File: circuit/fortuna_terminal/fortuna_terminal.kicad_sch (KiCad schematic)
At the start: 10 parts

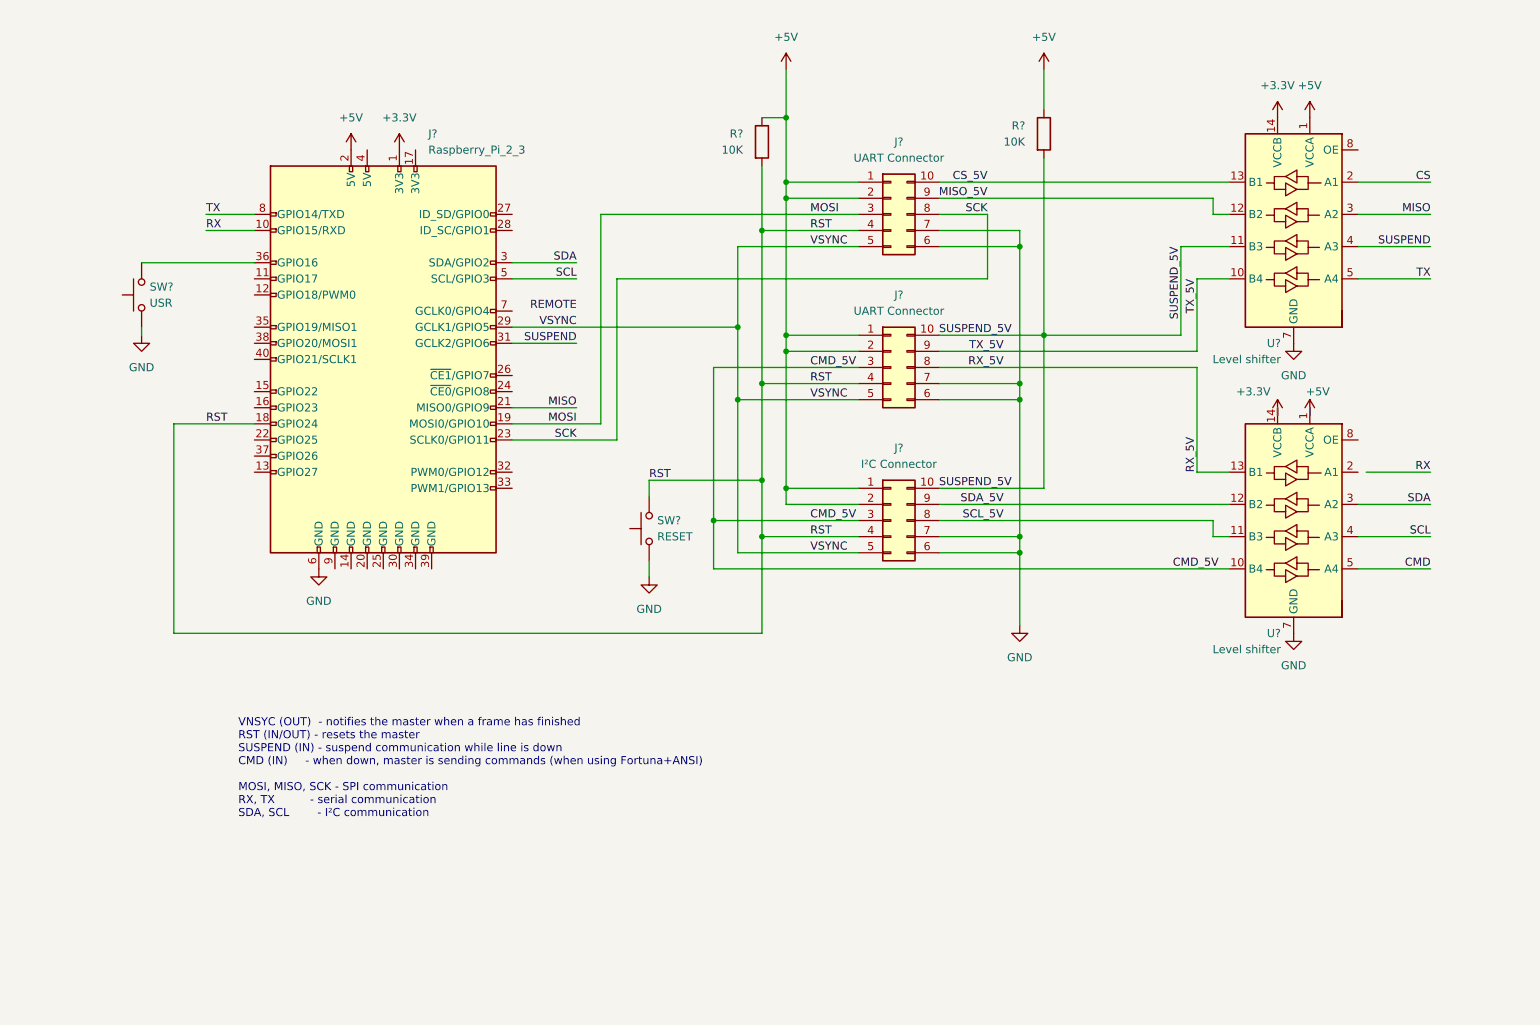
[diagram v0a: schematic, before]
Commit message: WIP
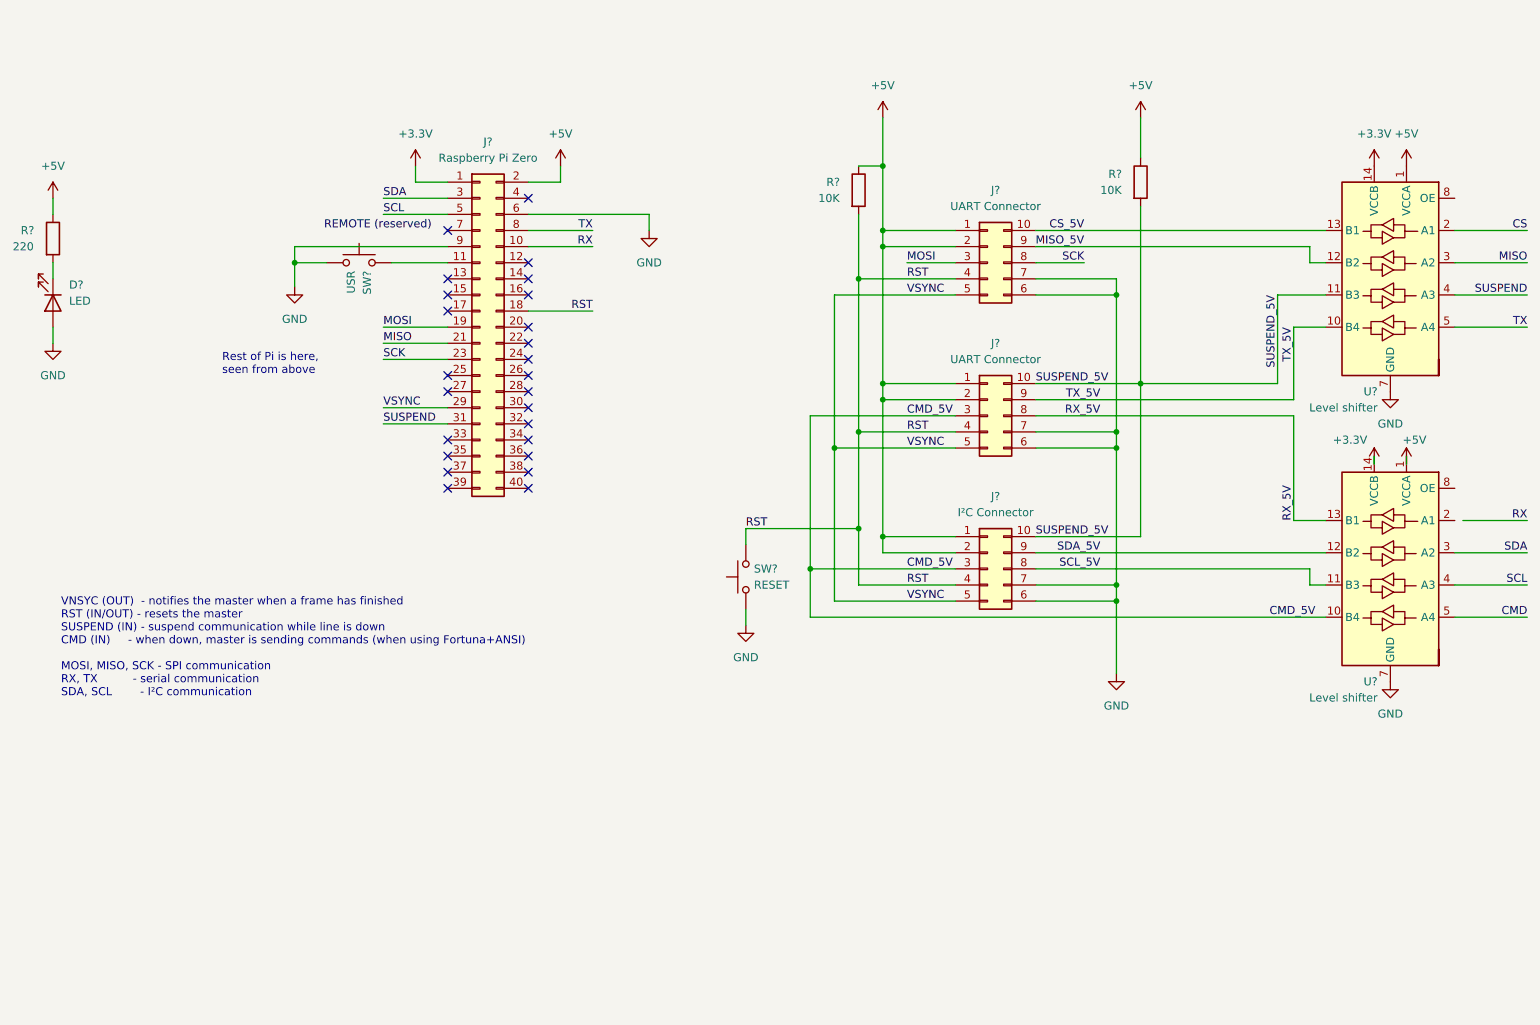
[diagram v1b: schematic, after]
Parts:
- removed J?: Raspberry_Pi_2_3, symbol Connector:Raspberry_Pi_2_3
- removed SW?: USR, symbol Switch:SW_Push
- added D?: LED, symbol Device:LED
- added J?: Raspberry Pi Zero, symbol Connector_Generic:Conn_02x20_Odd_Even
- added R?: 220, symbol Device:R
- added SW?: USR, symbol Switch:SW_Push
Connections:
- net +3.3V: now also J?.1 (Pin_1)
- net +5V: now also J?.2 (Pin_2), R?.1
- net GND: now also D?.2 (A), J?.6 (Pin_6), J?.9 (Pin_9), SW?.1
- net MISO: now also J?.21 (Pin_21)
- net MOSI: now also J?.19 (Pin_19)
- net RST: now also J?.18 (Pin_18)
- net RX: now also J?.10 (Pin_10)
- net SCK: now also J?.23 (Pin_23)
- net SCL: now also J?.5 (Pin_5)
- net SDA: now also J?.3 (Pin_3)
- net SUSPEND: now also J?.31 (Pin_31)
- net TX: now also J?.8 (Pin_8)
- net VSYNC: now also J?.29 (Pin_29)
- new net: J?.11 (Pin_11), SW?.2
- new net: D?.1 (K), R?.2
- no-connect marks 0 -> 25
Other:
- note added: "Rest of Pi is here, seen from above"
- moved on the sheet: J?, R?, SW?, U?

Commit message: WIP
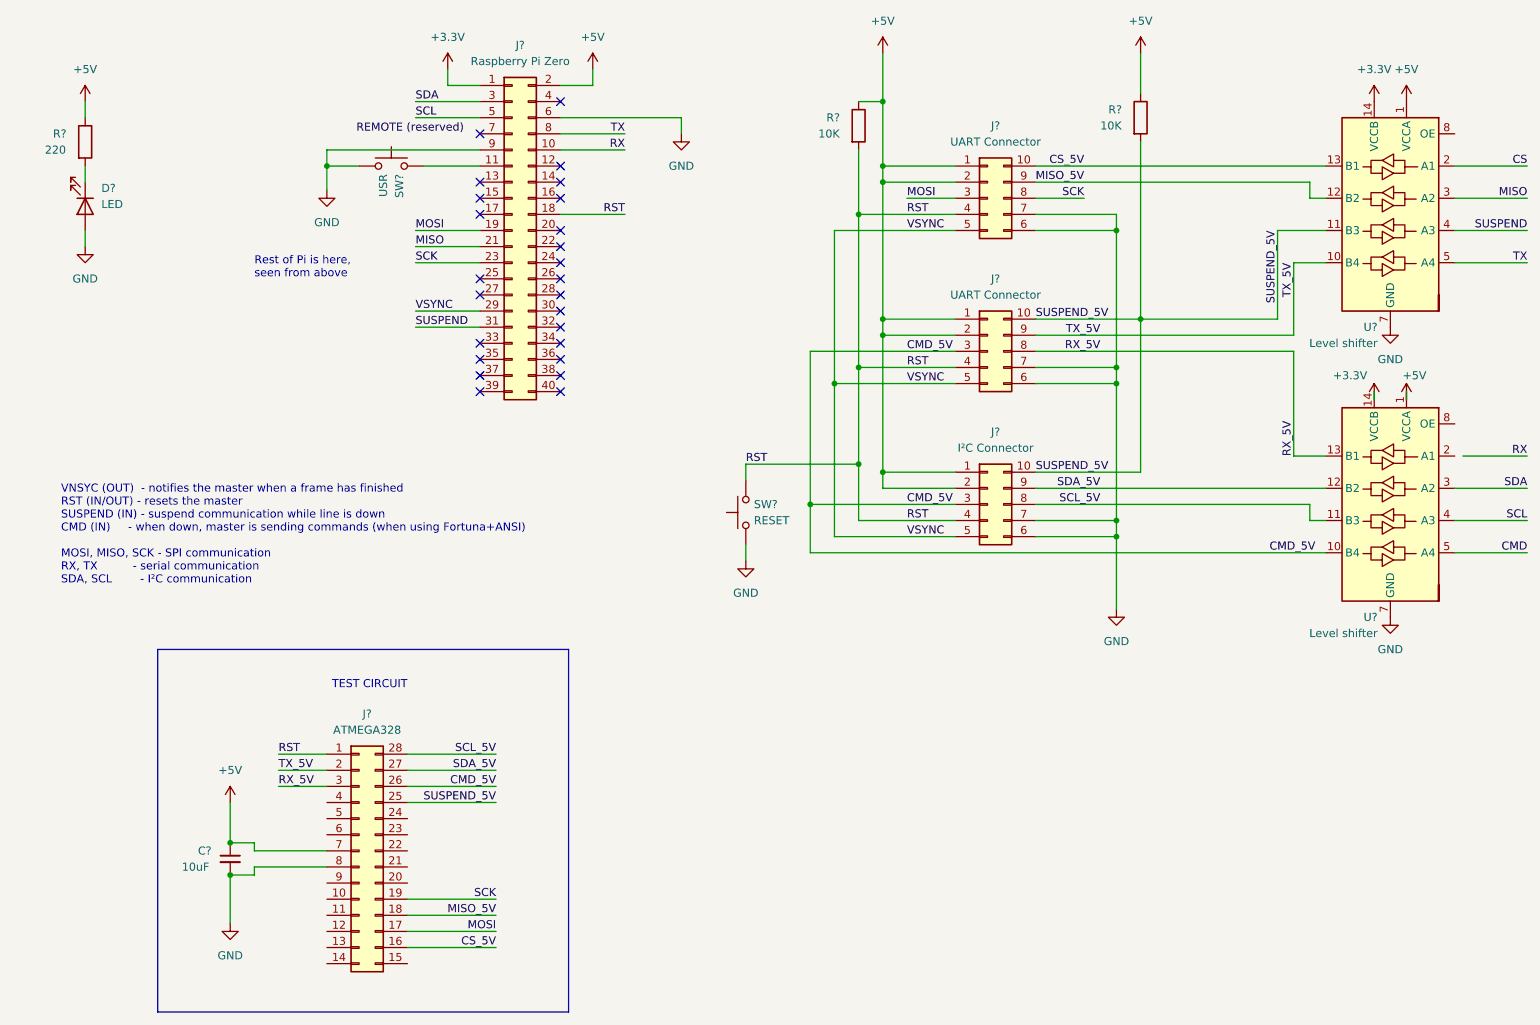
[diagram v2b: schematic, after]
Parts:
- added C?: 10uF, symbol Device:C_Small
- added J?: ATMEGA328, symbol Connector_Generic:Conn_02x14_Counter_Clockwise
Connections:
- net +5V: now also C?.1, J?.7 (Pin_7)
- net CMD_5V: now also J?.26 (Pin_26)
- net CS_5V: now also J?.16 (Pin_16)
- net GND: now also C?.2, J?.8 (Pin_8)
- net MISO_5V: now also J?.18 (Pin_18)
- net MOSI: now also J?.17 (Pin_17)
- net RST: now also J?.1 (Pin_1)
- net RX_5V: now also J?.3 (Pin_3)
- net SCK: now also J?.19 (Pin_19)
- net SCL_5V: now also J?.28 (Pin_28)
- net SDA_5V: now also J?.27 (Pin_27)
- net SUSPEND_5V: now also J?.25 (Pin_25)
- net TX_5V: now also J?.2 (Pin_2)
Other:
- note added: "TEST CIRCUIT"
- moved on the sheet: D?, J?, R?, SW?, U?
